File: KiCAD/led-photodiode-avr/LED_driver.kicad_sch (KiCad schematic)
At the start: 18 parts, among them Q1 TTC1949, Q2 TTC1949, Q3 TTC1949, Q4 TTC1949, U6 LTC1380, U8 OPA365AIDR, U9 LTC2631

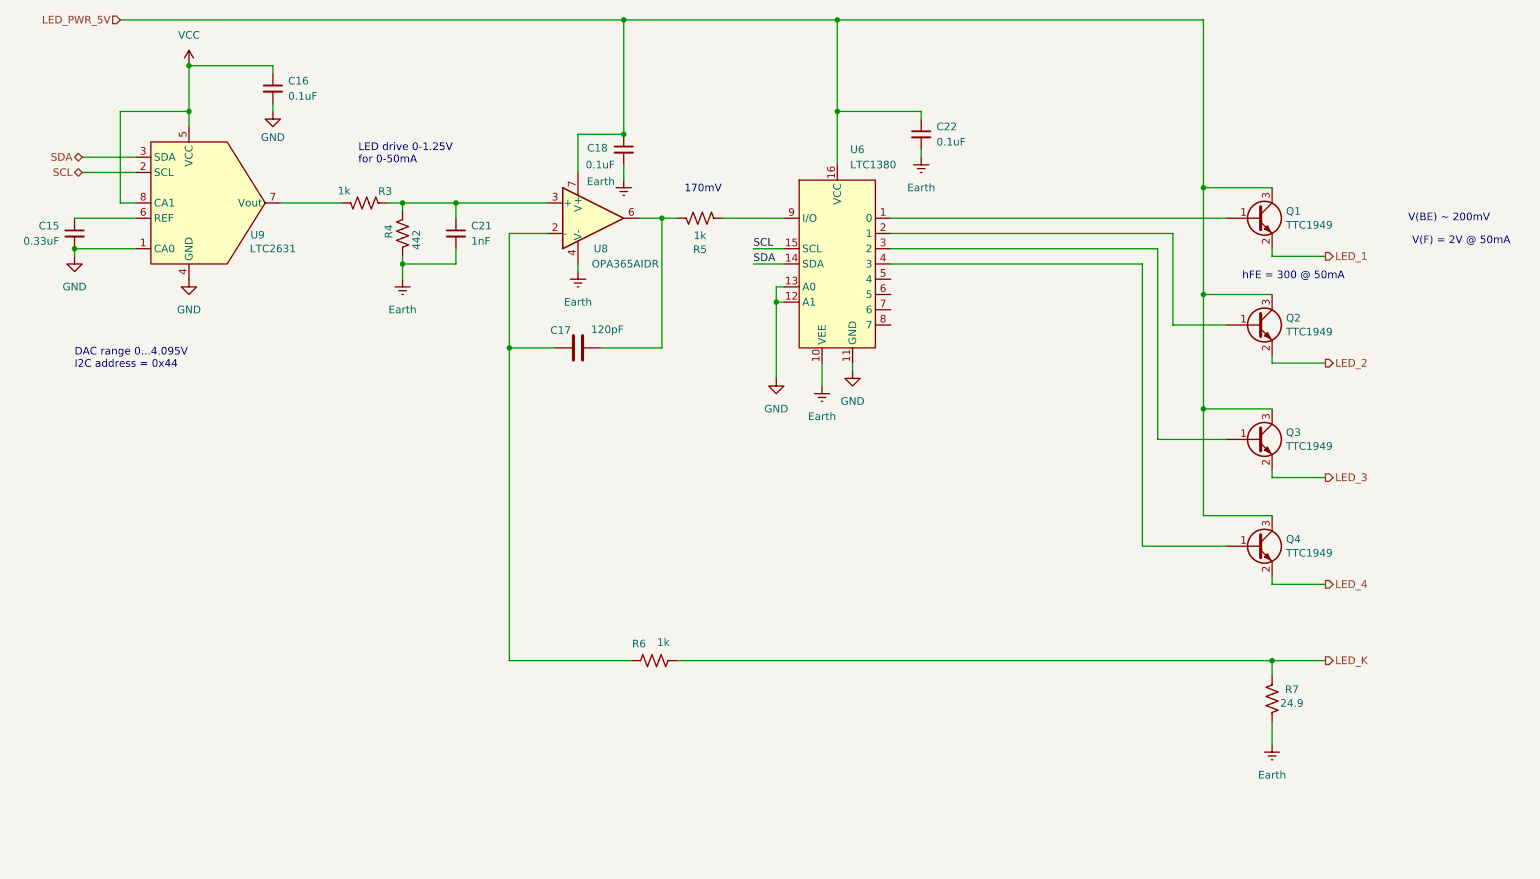
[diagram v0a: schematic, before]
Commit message: starting on V2
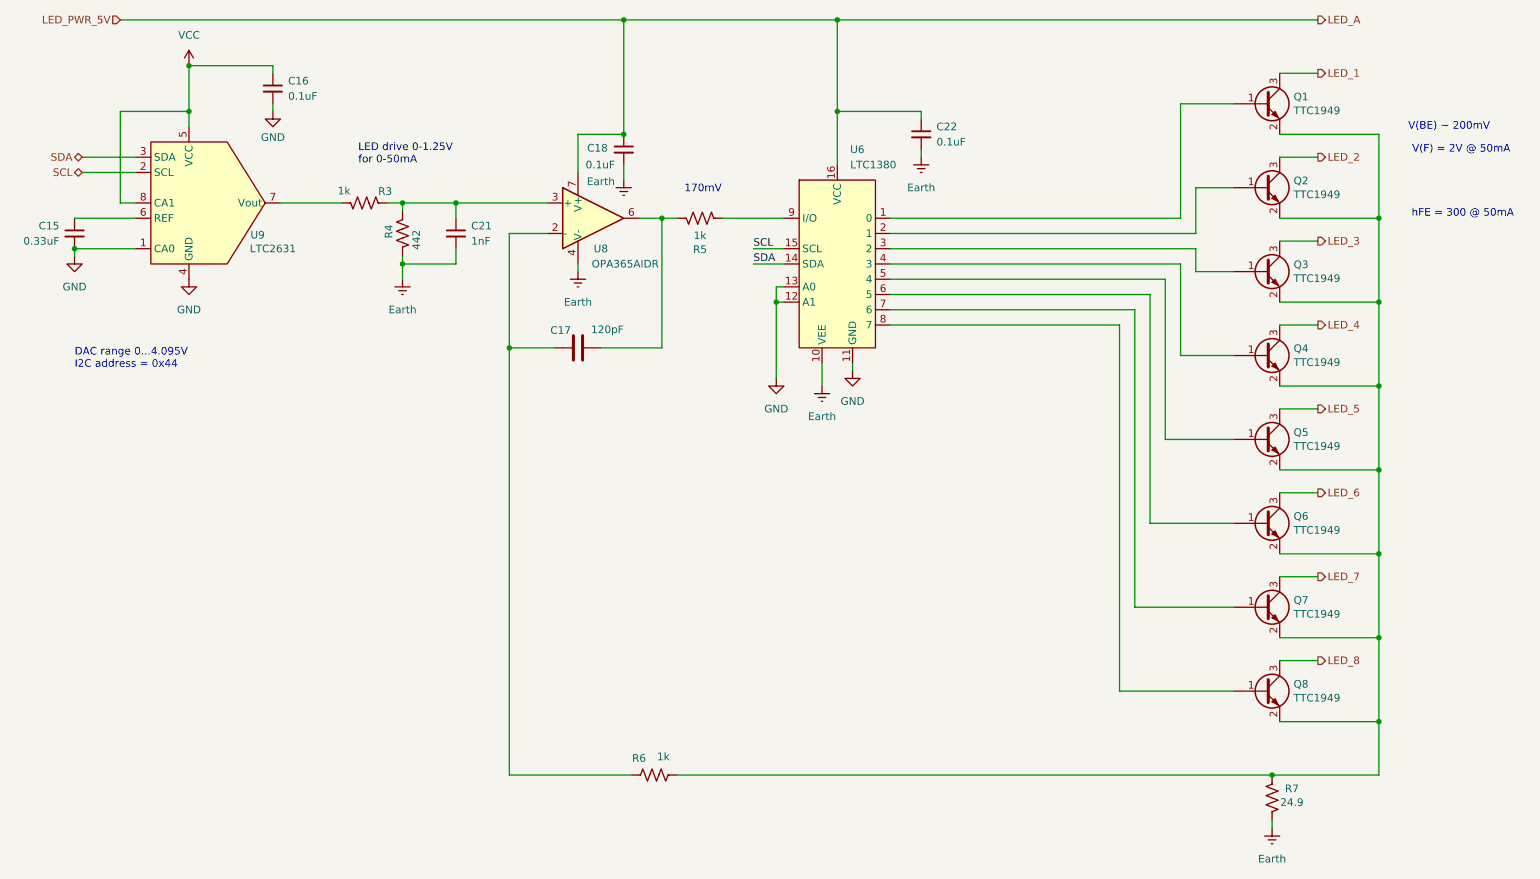
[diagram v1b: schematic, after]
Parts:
- added Q5, Q6, Q7, Q8: TTC1949, Package_TO_SOT_SMD:SC-59, symbol my_BJT:TTC1949
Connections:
- net LED_1: now also Q1.3 (C); no longer Q1.2 (E)
- net LED_2: now also Q2.3 (C); no longer Q2.2 (E)
- net LED_3: now also Q3.3 (C); no longer Q3.2 (E)
- net LED_4: now also Q4.3 (C); no longer Q4.2 (E)
- net at U6.5 (4): now also Q5.1 (B)
- net at U6.6 (5): now also Q6.1 (B)
- net at U6.7 (6): now also Q7.1 (B)
- net at U6.8 (7): now also Q8.1 (B)
- net LED_K: no longer names the net of R6.1, R7.2
- net LED_K: now also Q1.2 (E), Q2.2 (E), Q3.2 (E), Q4.2 (E), Q5.2 (E), Q6.2 (E), Q7.2 (E), Q8.2 (E)
- net LED_PWR_5V renamed LED_A
- net LED_A: no longer Q1.3 (C), Q2.3 (C), Q3.3 (C), Q4.3 (C)
- new net LED_5: Q5.3 (C)
- new net LED_6: Q6.3 (C)
- new net LED_7: Q7.3 (C)
- new net LED_8: Q8.3 (C)
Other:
- moved on the sheet: Q1, Q2, Q3, Q4, R6, R7
